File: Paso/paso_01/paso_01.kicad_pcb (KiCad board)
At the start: 2 copper layers, 97.4 x 87.2 mm, 2 parts

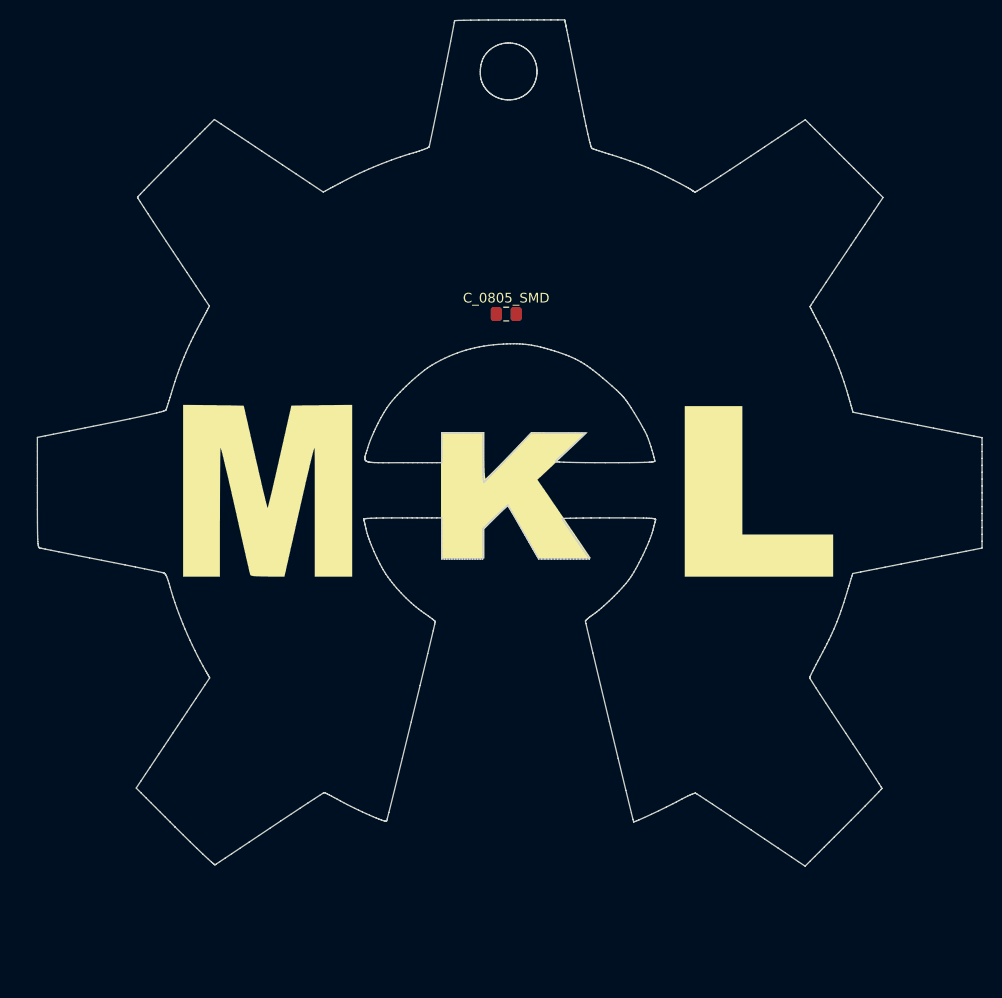
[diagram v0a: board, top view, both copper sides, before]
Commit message: Some minors update paso
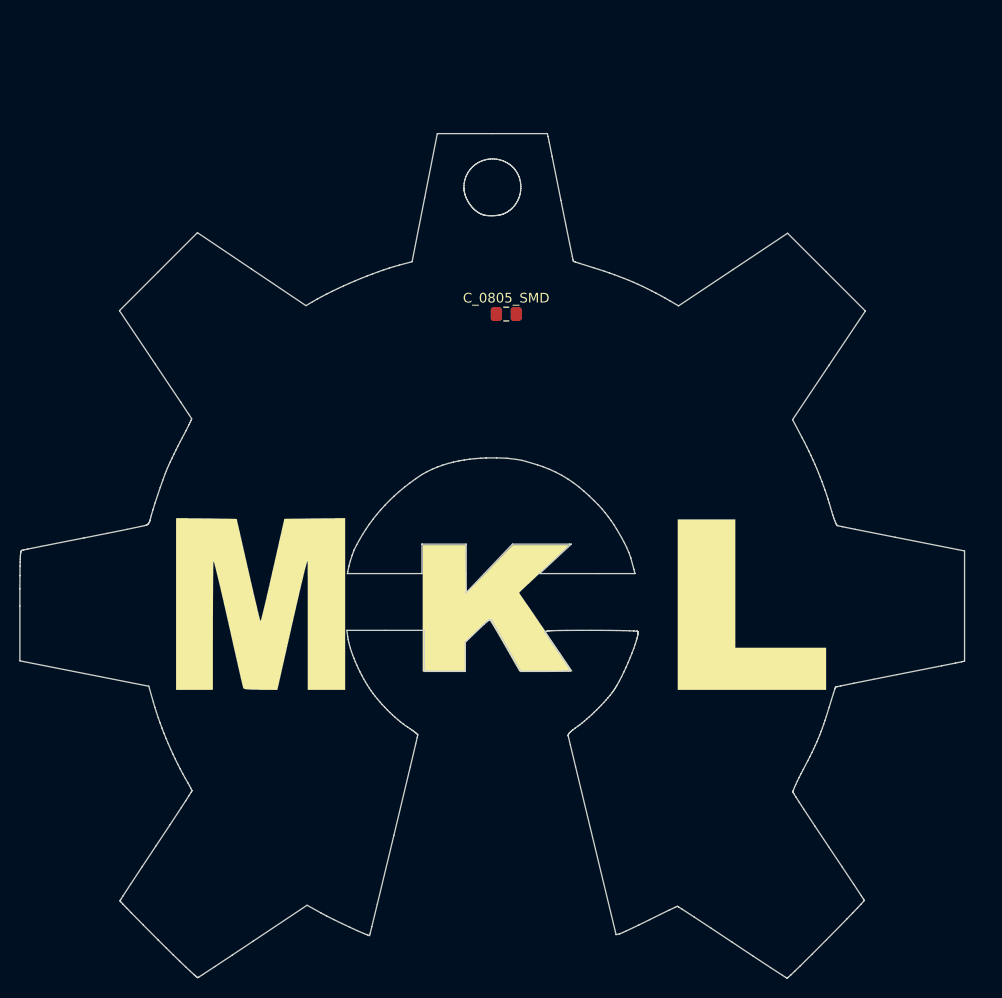
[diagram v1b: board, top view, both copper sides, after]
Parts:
- removed the Ref** at (117.0, 110.7)
- added Ref**: Val**, paso_01:Maker_Lugo_100mm_02, F.Cu at (116.3, 122.3)
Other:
- board size 97.4 x 87.2 mm -> 97.4 x 87 mm
